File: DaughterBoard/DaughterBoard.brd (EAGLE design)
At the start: 26.5 x 54.5 mm, 22 parts

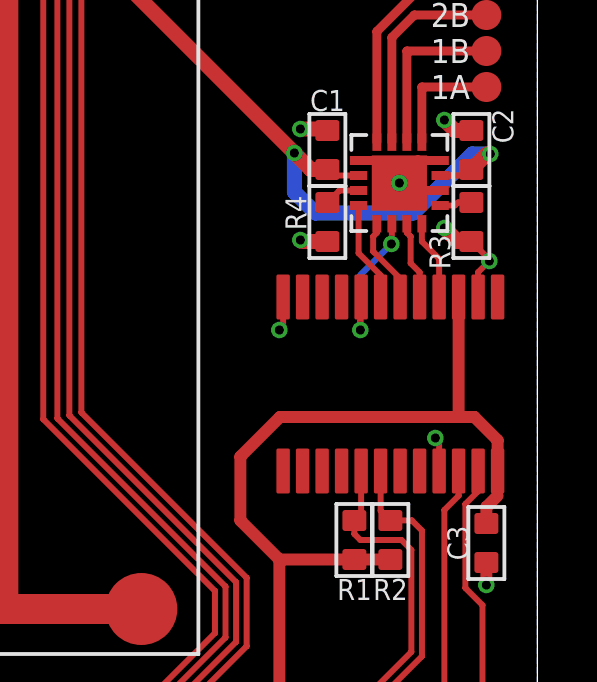
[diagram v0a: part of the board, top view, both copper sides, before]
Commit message: looks better
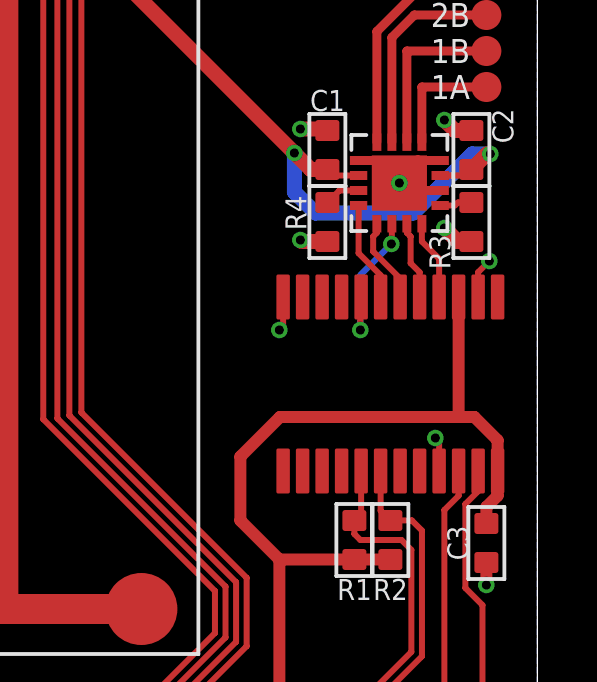
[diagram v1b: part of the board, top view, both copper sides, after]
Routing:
- net GND: track 56.4 -> 55.2 mm
- net +3.3V: track 57.7 -> 58.5 mm
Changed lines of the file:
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@@
 <contactref element="C1" pad="B"/>
 <contactref element="C2" pad="A"/>
-<wire x1="11.51305" y1="12.1" x2="11.2" y2="12.1" width="0.2" layer="1"/>
 <wire x1="10.45" y1="12.85" x2="9.84" y2="12.85" width="0.3" layer="1"/>
 <wire x1="12.56" y1="11.85" x2="11.45" y2="11.85" width="0.3" layer="1"/>
@@
 <wire x1="7.325" y1="7.325" x2="7.2" y2="7.2" width="0.2" layer="1"/>
 <via x="7.2" y="7.2" extent="1-16" drill="0.3"/>
-<wire x1="13.6" y1="10.15" x2="14.2" y2="9.55" width="0.2" layer="1"/>
-<wire x1="14.2" y1="9.55" x2="14.2" y2="9.5" width="0.2" layer="1"/>
 <via x="14.2" y="9.5" extent="1-16" drill="0.3"/>
 <wire x1="13.825" y1="8.3" x2="13.825" y2="9.125" width="0.2" layer="1"/>
@@
 <wire x1="5.9" y1="0.85" x2="7.2" y2="-0.45" width="0.4" layer="1"/>
 <wire x1="14.1" y1="1.3" x2="14.1" y2="0.75" width="0.4" layer="1"/>
-<wire x1="14.475" y1="1.675" x2="14.1" y2="1.3" width="0.4" layer="1"/>
 <wire x1="7.2205" y1="4.3" x2="5.9" y2="2.9795" width="0.4" layer="1"/>
 <wire x1="5.9" y1="2.9795" x2="5.9" y2="0.85" width="0.4" layer="1"/>
@@
 <wire x1="13.175" y1="4.3" x2="7.2205" y2="4.3" width="0.4" layer="1"/>
 <wire x1="13.175" y1="8.3" x2="13.175" y2="4.3" width="0.4" layer="1"/>
-<wire x1="14.475" y1="2.5" x2="14.475" y2="1.675" width="0" layer="19" extent="1-1"/>
+<wire x1="14.475" y1="2.5" x2="14.475" y2="1.675" width="0.4" layer="1"/>
+<wire x1="14.475" y1="1.675" x2="14.1" y2="1.3" width="0.4" layer="1"/>
 </signal>
 <signal name="N$1">
